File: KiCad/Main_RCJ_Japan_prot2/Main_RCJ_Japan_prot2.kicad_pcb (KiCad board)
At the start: 2 copper layers, 73.7 x 73.6 mm, 20 parts, among them J1 Conn_01x04_Socket, J2 Conn_01x04_Socket, J3 Conn_01x04_Socket, J4 Conn_01x04_Socket, J5 Conn_01x04_Socket, J6 Conn_01x04_Socket, J7 Conn_01x02_Socket, J8 Conn_01x06_Socket, SW1 SW_Push

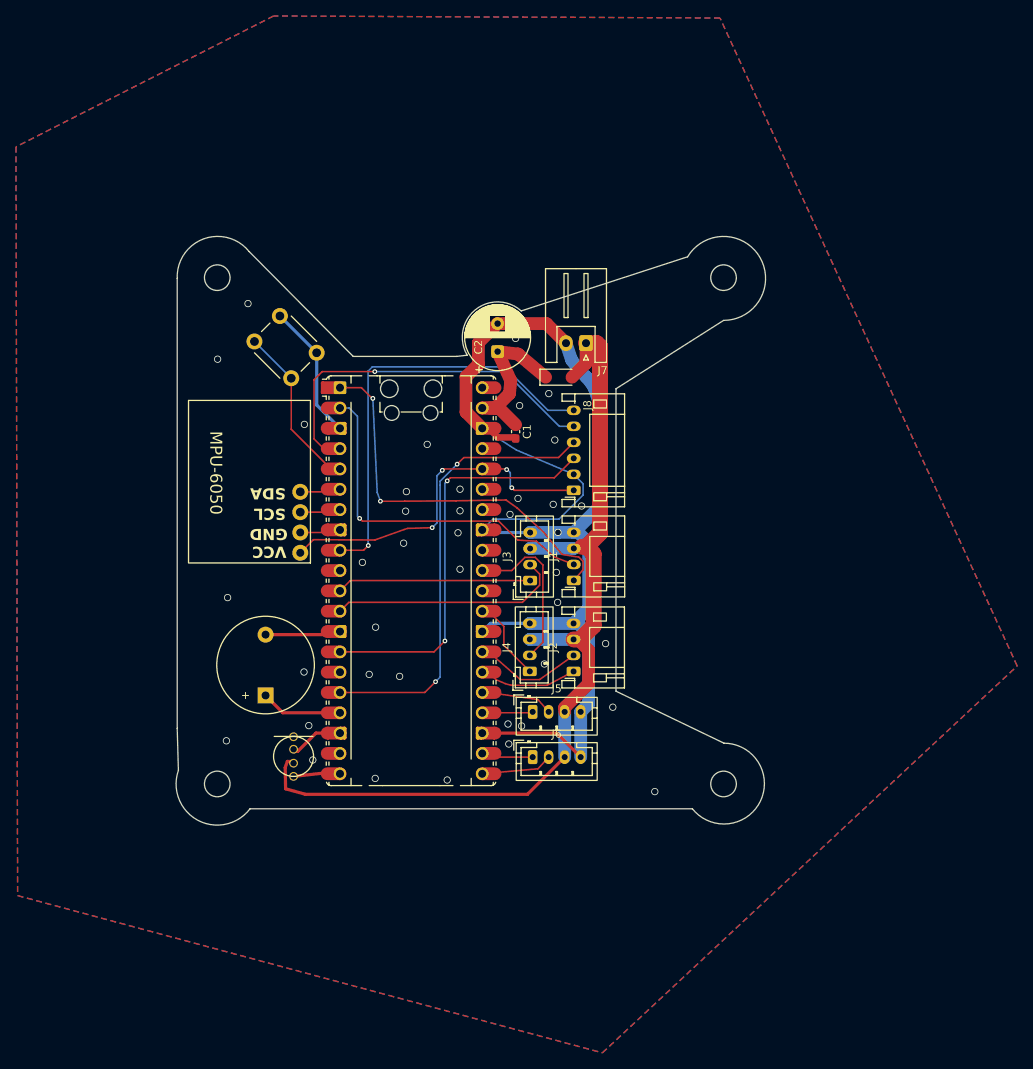
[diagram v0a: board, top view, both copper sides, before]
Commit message: 新メイン完成
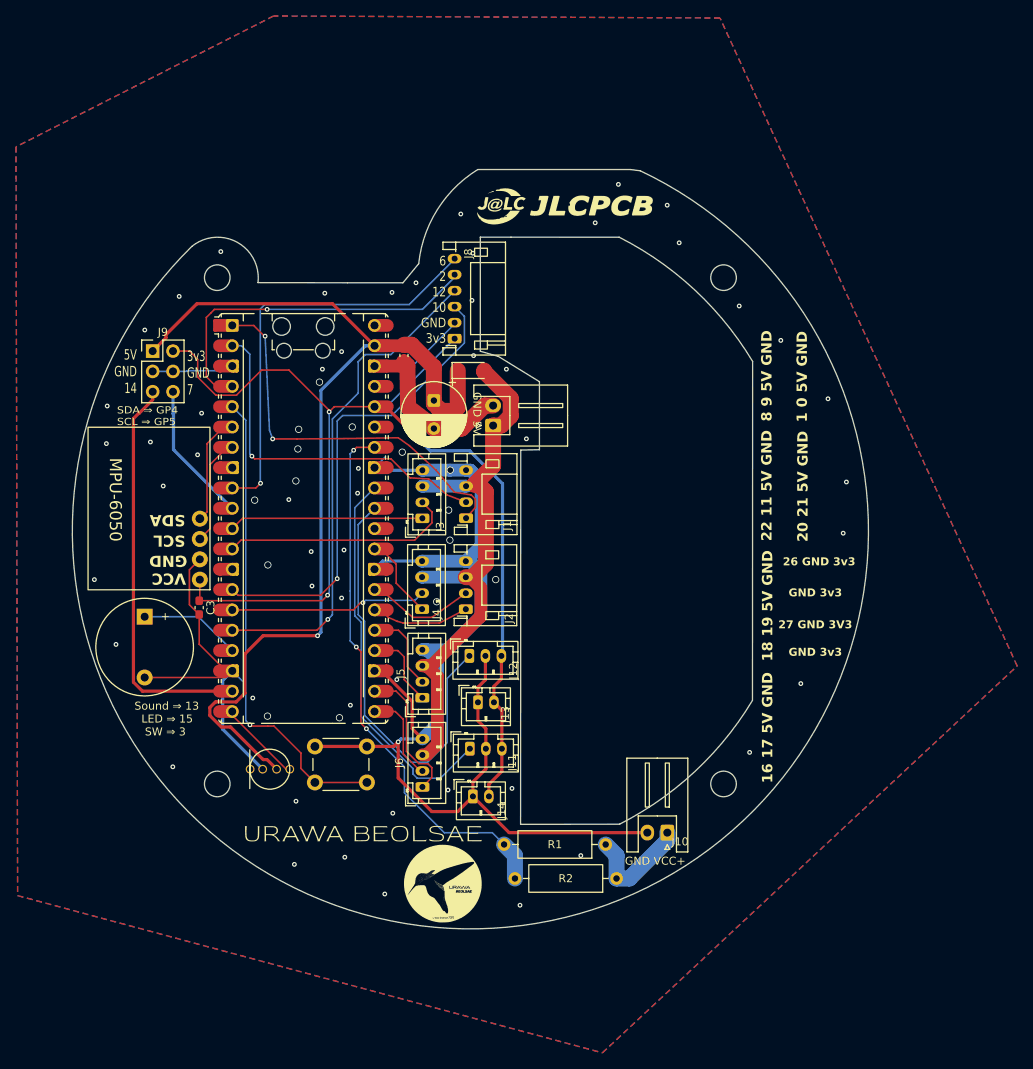
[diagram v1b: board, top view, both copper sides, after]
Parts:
- added C3: C, Capacitor_SMD:C_0603_1608Metric_Pad1.08x0.95mm_HandSolder, F.Cu at (66.1, 109.6)
- added G***: LOGO, LOGO:名称未設定, F.Cu at (86.5, 137.8)
- added G***: LOGO, LOGO:ICON, F.Cu at (96.6, 144.1)
- added G***: LOGO, LOGO:logo, F.Cu at (111.7, 59.4)
- added J10: Conn_01x02_Socket, Connector_JST:JST_XH_S2B-XH-A_1x02_P2.50mm_Horizontal, F.Cu at (124.6, 137.7)
- added J11: Conn_01x03_Socket, Connector_JST:JST_PH_B3B-PH-K_1x03_P2.00mm_Vertical, F.Cu at (99.9, 127.2)
- added J12: Conn_01x03_Socket, Connector_JST:JST_PH_B3B-PH-K_1x03_P2.00mm_Vertical, F.Cu at (99.9, 115.6)
- added J13: Conn_01x02_Socket, Connector_JST:JST_PH_B2B-PH-K_1x02_P2.00mm_Vertical, F.Cu at (100.9, 121.4)
- added J14: Conn_01x02_Socket, Connector_JST:JST_PH_B2B-PH-K_1x02_P2.00mm_Vertical, F.Cu at (100.3, 133.2)
- added J9: Conn_02x03_Odd_Even, Connector_PinHeader_2.54mm:PinHeader_2x03_P2.54mm_Vertical, F.Cu at (60.3, 77.5)
- added R1: R, Resistor_THT:R_Axial_DIN0309_L9.0mm_D3.2mm_P12.70mm_Horizontal, F.Cu at (116.9, 139.2)
- added R2: R, Resistor_THT:R_Axial_DIN0309_L9.0mm_D3.2mm_P12.70mm_Horizontal, F.Cu at (118.3, 143.5)
- moved SW1 54.0 mm to (80.6, 127.0), turned to 0 degrees
- moved J8 24.1 mm to (98.0, 76.0)
- moved BZ1 18.0 mm to (59.3, 110.7), turned to -90 degrees
- moved C1 16.9 mm to (91.7, 78.1)
- moved J3 15.6 mm to (94.0, 98.4)
- moved A1 15.6 mm to (79.1, 98.5)
- moved J1 15.6 mm to (99.5, 98.4)
- moved J2 15.6 mm to (99.4, 109.8)
- moved J4 15.6 mm to (94.0, 109.8)
- moved J7 15.5 mm to (102.8, 86.8), turned to 90 degrees
- moved J6 14.3 mm to (94.0, 132.0), turned to 90 degrees
- moved J5 13.9 mm to (94.0, 120.9), turned to 90 degrees
- moved U1 13.0 mm to (61.1, 101.0)
- moved D2 11.0 mm to (100.1, 80.0)
- moved C2 10.0 mm to (95.4, 83.7), turned to -90 degrees
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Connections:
- A1 pad 10: unconnected-(A1-GPIO7-Pad10) -> Net-(A1-GPIO7)
- A1 pad 15: unconnected-(A1-GPIO11-Pad15) -> PIO-UART1_RX
- A1 pad 19: unconnected-(A1-GPIO14-Pad19) -> Net-(A1-GPIO14)
- A1 pad 31: PIO-UART1_RX -> ADC1
- A1 pad 32: unconnected-(A1-GPIO27_ADC1-Pad32) -> ADC2
- A1 pad 34: unconnected-(A1-GPIO28_ADC2-Pad34) -> BATT_ADC
- U2 pad 3: VCC -> Net-(A1-VSYS)
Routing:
- net 3v3: track 43.7 -> 148.9 mm, vias 4 -> 3
- net Net-(A1-VSYS): track 21.1 -> 126.0 mm, vias 0 -> 1
- net BATT_ADC: track 0.00 -> 68.5 mm, vias 0 -> 3
- net ADC1: track 0.00 -> 52.8 mm
- net GND: track 193.3 -> 245.9 mm, vias 40 -> 69
- net Net-(A1-GPIO14): track 0.00 -> 49.4 mm
- net ADC2: track 0.00 -> 48.6 mm
- net VCC: track 115.8 -> 72.3 mm
- net Net-(A1-GPIO3): track 21.0 -> 59.4 mm, vias 0 -> 1
- net Net-(A1-GPIO7): track 0.00 -> 17.6 mm
- net Net-(J10-Pin_1): track 0.00 -> 14.1 mm
- net SDA: track 4.30 -> 15.4 mm
- net PIO-UART3_TX: track 6.50 -> 17.5 mm
- net SCL: track 4.30 -> 14.0 mm
- net kicker_in1: track 50.8 -> 59.0 mm, vias 2 -> 1
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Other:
- board size 73.7 x 73.6 mm -> 99.5 x 94.9 mm
- board text added: "+ -"
- board text added: "- +"
- board text added: "1 0 5V GND"
- board text added: "16 17 5V GND"
- board text added: "18 19 5V GND"
- board text added: "20 21 5V GND"
- board text added: "22 11 5V GND"
- board text added: "26 GND 3v3"
- board text added: "27 GND 3V3"
- board text added: "3v3 GND 7"
- board text added: "5V GND 14"
- board text added: "6 2 12 10 GND 3v3"
- board text added: "8 9 5V GND"
- board text added: "GND 3v3"
- board text added: "GND 5V"
- board text added: "GND VCC+"
- board text added: "SDA ⇒ GP4 SCL ⇒ GP5"
- board text added: "Sound ⇒ 13 LED ⇒ 15 SW ⇒ 3"
